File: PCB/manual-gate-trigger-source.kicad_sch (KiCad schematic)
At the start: 57 parts

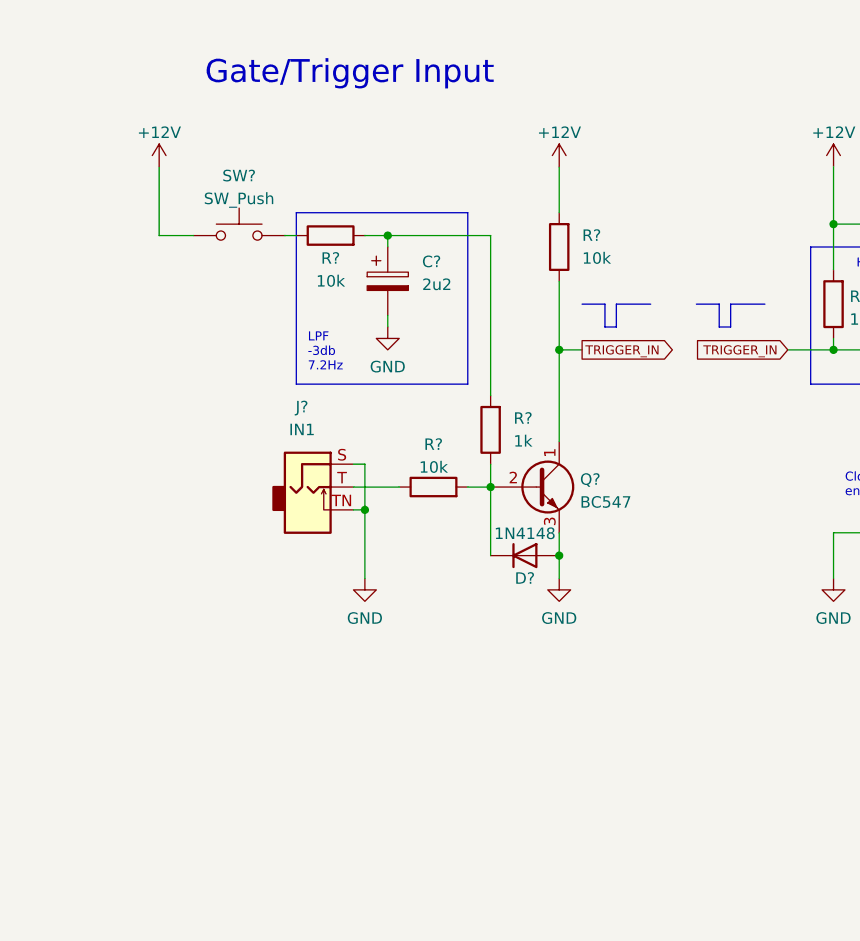
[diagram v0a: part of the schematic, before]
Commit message: :hammer: separate input into manual and CV
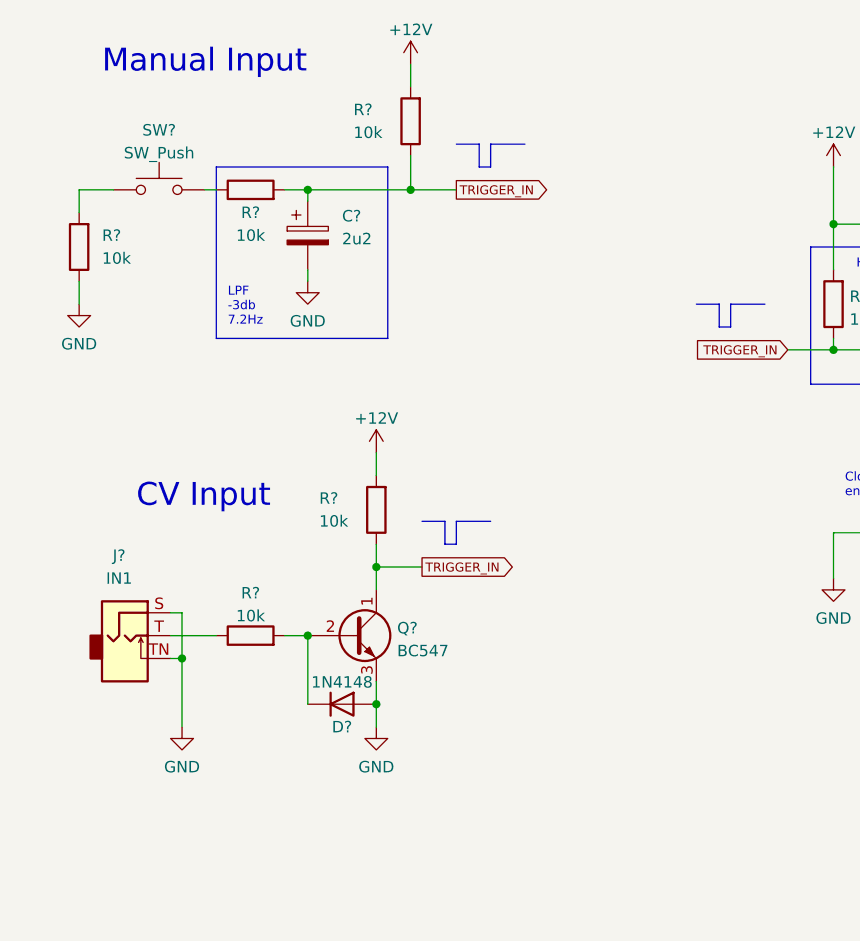
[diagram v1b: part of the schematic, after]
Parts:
- removed R?: 1k, symbol Device:R
- added R? (x2): 10k, symbol Device:R
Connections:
- net +12V: now also R?.2; no longer SW?.1
- net GND: now also R?.1
- net TRIGGER_IN: now also C?.1, R?.2, R?.1
- new net: R?.2, SW?.1
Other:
- note added: "CV Input"
- note added: "Manual Input"
- note removed: "Gate/Trigger Input"
- moved on the sheet: C?, D?, J?, Q?, R?, SW?
